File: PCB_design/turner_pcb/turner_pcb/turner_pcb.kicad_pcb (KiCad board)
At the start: 2 copper layers, 2 parts, among them U1 TMC2208_SILENTSTEPSTICK

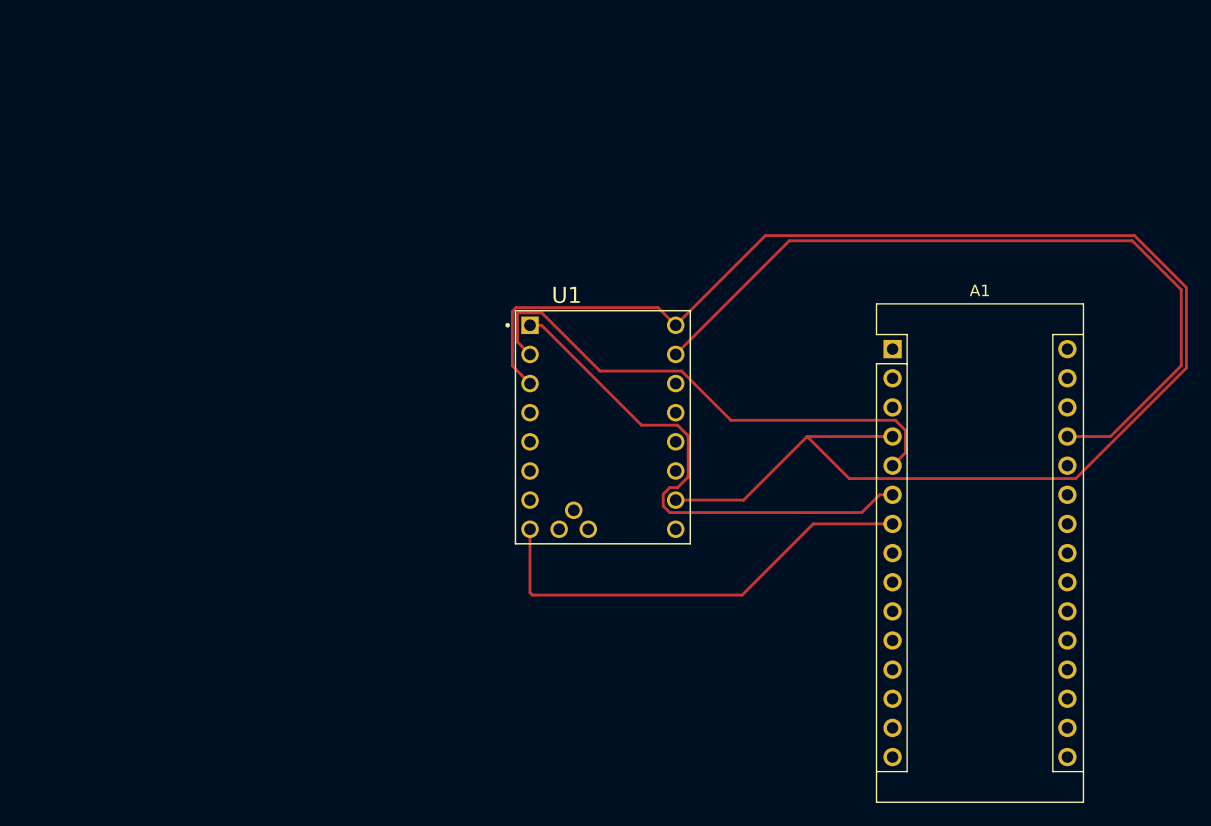
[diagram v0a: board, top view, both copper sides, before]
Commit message: first complete version on pcb
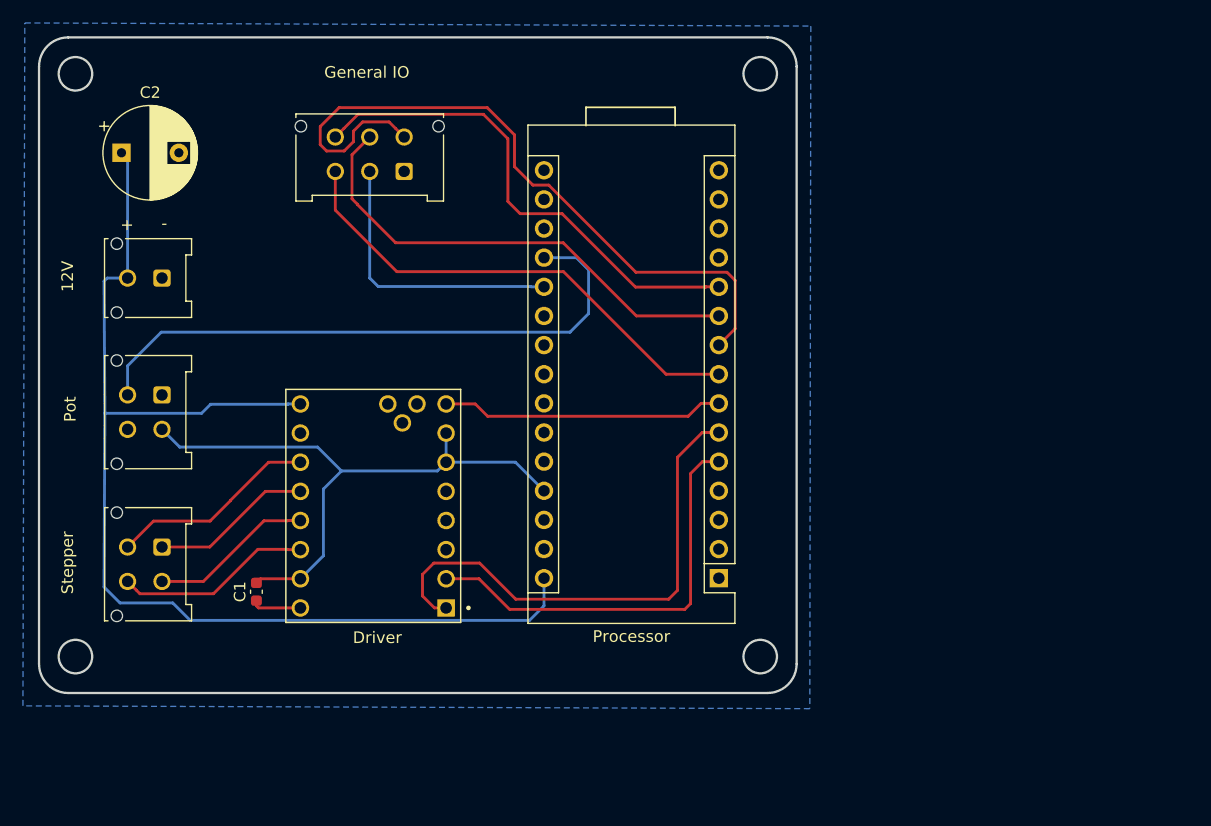
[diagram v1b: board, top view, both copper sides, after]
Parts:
- removed U1: TMC2208_SILENTSTEPSTICK, TMC2208_SILENTSTEPSTICK:MODULE_TMC2208_SILENTSTEPSTICK
- added 12V: Conn_01x02, Connector_Molex:Molex_Micro-Fit_3.0_43045-0212_2x01_P3.00mm_Vertical, F.Cu at (55.7, 42.9)
- added C1: C_Small, Capacitor_SMD:C_0603_1608Metric, F.Cu at (63.9, 70.2)
- added C2: C_Polarized, Capacitor_THT:CP_Radial_D8.0mm_P5.00mm, F.Cu at (52.2, 32.0)
- added Driver: TMC2208_SILENTSTEPSTICK, TMC2208_SILENTSTEPSTICK:MODULE_TMC2208_SILENTSTEPSTICK, F.Cu at (74.1, 62.8)
- added General IO: Conn_02x03_Odd_Even, Connector_Molex:Molex_Micro-Fit_3.0_43045-0612_2x03_P3.00mm_Vertical, F.Cu at (76.8, 33.6)
- added Pot: Conn_02x02_Odd_Even, Connector_Molex:Molex_Micro-Fit_3.0_43045-0412_2x02_P3.00mm_Vertical, F.Cu at (55.7, 53.1)
- added Stepper: Conn_02x02_Odd_Even, Connector_Molex:Molex_Micro-Fit_3.0_43045-0412_2x02_P3.00mm_Vertical, F.Cu at (55.7, 66.3)
- moved Processor 25.1 mm to (104.2, 69.1), turned to 180 degrees
- renumbered A1 to Processor
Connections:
- Processor pad 10: Net-(A1-Pad10) -> DIO3
- Processor pad 11: Net-(A1-Pad11) -> DIO4
- Processor pad 19: Net-(A1-Pad19) -> Pot
- Processor pad 20: Net-(A1-Pad20) -> AO1
- Processor pad 30: Net-(A1-Pad30) -> +12V
- Processor pad 8: Net-(A1-Pad8) -> DIO1
- Processor pad 9: Net-(A1-Pad9) -> DIO2
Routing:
- net GND: track 138.3 -> 4.36 mm
- net +12V: track 0.00 -> 100.6 mm
- net DIO2: track 0.00 -> 62.2 mm
- net Pot: track 0.00 -> 52.7 mm
- net DIO4: track 0.00 -> 43.7 mm
- net DIO1: track 0.00 -> 42.7 mm
- net DIO3: track 0.00 -> 42.3 mm
- net AO1: track 0.00 -> 24.8 mm
- net DA2: track 0.00 -> 18.1 mm
- net DB2: track 0.00 -> 17.1 mm
- net +5V: track 69.0 -> 53.6 mm
- net Enable: track 39.8 -> 24.7 mm
- net DB1: track 0.00 -> 14.3 mm
- net DA1: track 0.00 -> 14.1 mm
- net Step: track 45.6 -> 36.8 mm
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- added copper zone on B.Cu, net GND
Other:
- board outline added: 66 x 57.1 mm
- board text added: "+"
- board text added: "-"
